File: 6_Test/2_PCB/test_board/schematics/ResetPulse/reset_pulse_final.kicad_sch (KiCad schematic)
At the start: 3 parts, among them J10 TSM-102-01-L-DV-P-TR

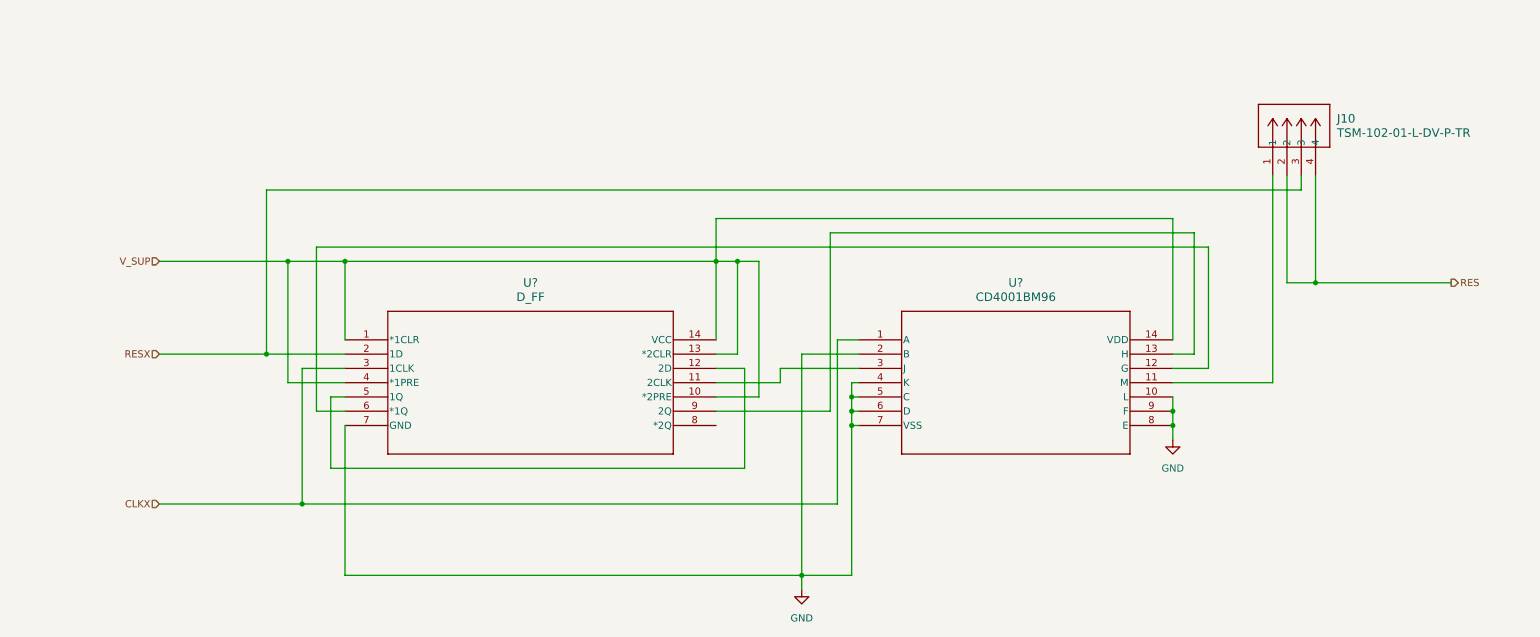
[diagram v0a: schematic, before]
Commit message: Adjusted Edits 11_25_24
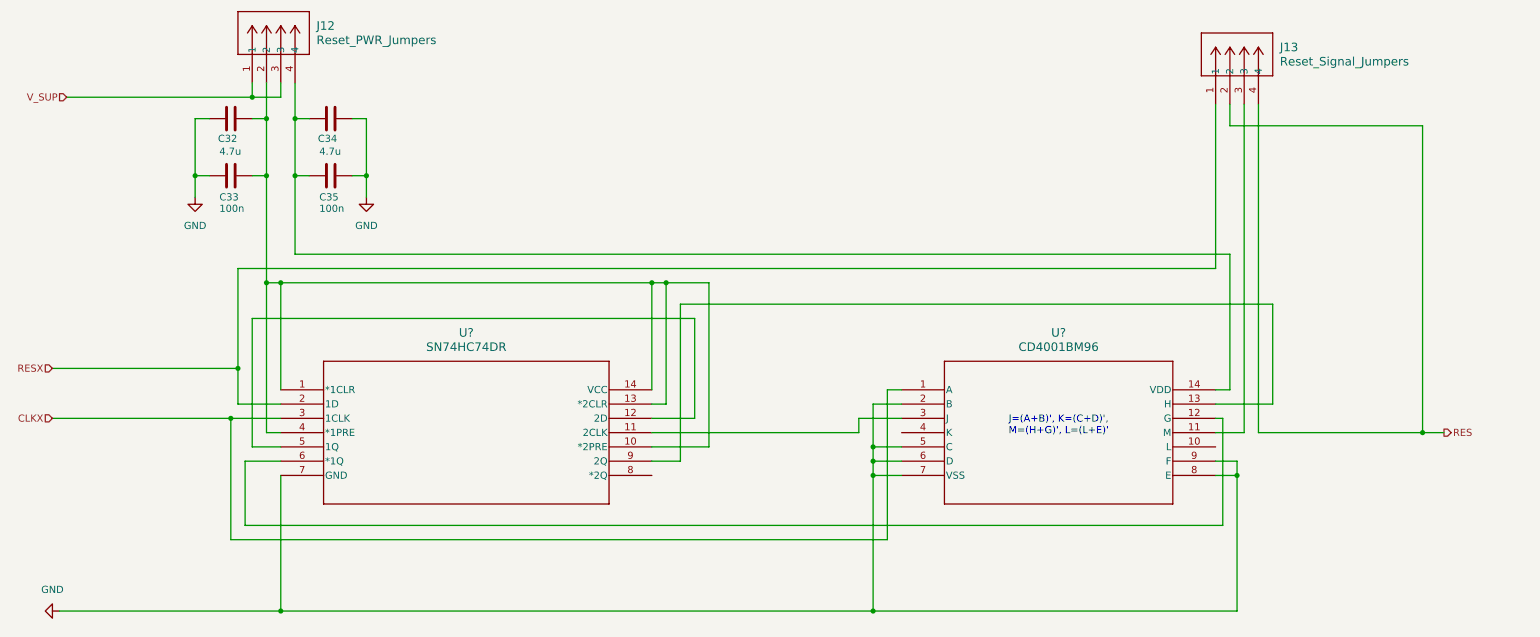
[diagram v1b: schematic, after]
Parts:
- added C32, C34: 4.7u, Capacitor_SMD:C_0603_1608Metric, symbol Device:C
- added C33, C35: 100n, Capacitor_SMD:C_0402_1005Metric, symbol Device:C
- added J12: Reset_PWR_Jumpers, CONN_TSM-102-01-L-DV-P-TR_SAI, symbol 2x2Header:TSM-102-01-L-DV-P-TR
- J13: renamed from J10; value TSM-102-01-L-DV-P-TR -> Reset_Signal_Jumpers
- U?: footprint nor_gate:nor_gate_D14 -> ECE628_lib:nor_gate_D14
- U?: value D_FF -> SN74HC74DR; footprint D14 -> ECE628_lib:flip_flop_D14
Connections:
- net GND: now also C32.2, C33.2, C34.1, C35.1; no longer U?.10 (L), U?.4 (K)
- net RESX: now also J13.1; no longer J13.3
- net V_SUP: now also J12.1, J12.3; no longer U?.1 (*1CLR), U?.10 (*2PRE), U?.13 (*2CLR), U?.14 (VCC), U?.14 (VDD), U?.4 (*1PRE)
- net at U?.11 (M): now also J13.3; no longer J13.1
- new net: C32.1, C33.1, J12.2, U?.1 (*1CLR), U?.10 (*2PRE), U?.13 (*2CLR), U?.14 (VCC), U?.4 (*1PRE)
- new net: C34.2, C35.2, J12.4, U?.14 (VDD)
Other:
- note added: "J=(A+B)', K=(C+D)', M=(H+G)', L=(L+E)'"
- moved on the sheet: J13, U?
